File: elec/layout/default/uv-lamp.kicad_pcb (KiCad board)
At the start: 2 copper layers, 21 x 21 mm, 3 parts, among them U1 ?, U2 ?, U3 ?

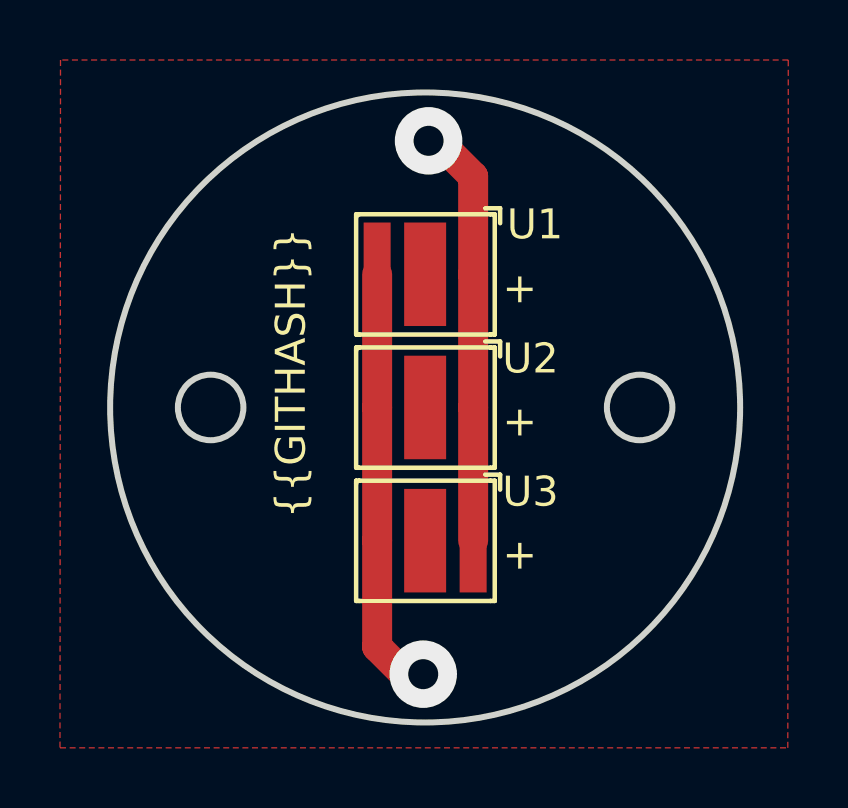
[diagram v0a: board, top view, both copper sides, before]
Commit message: readme
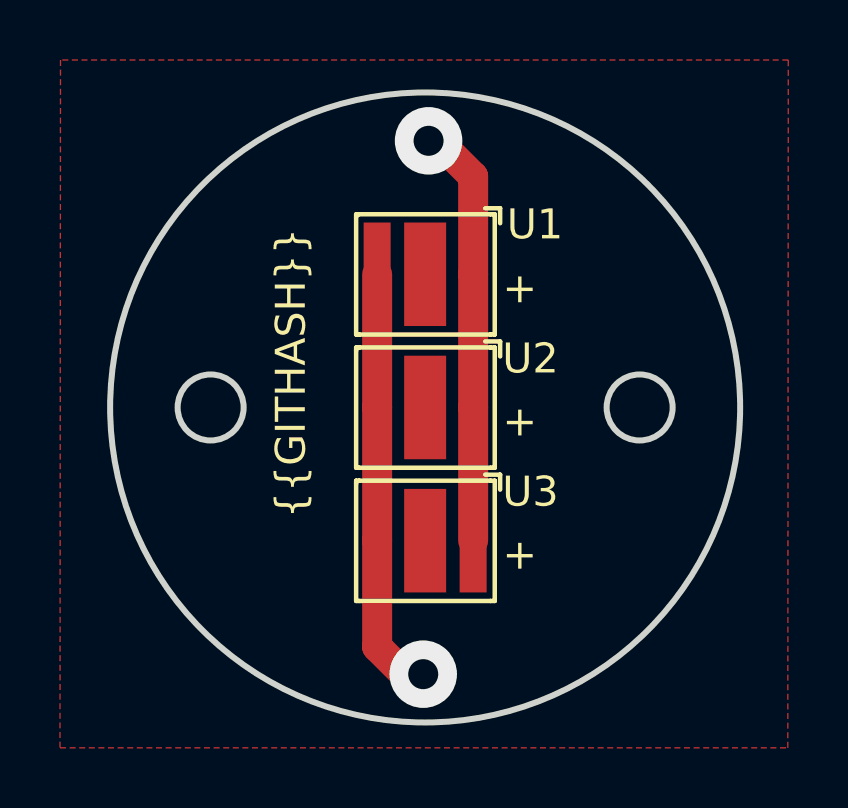
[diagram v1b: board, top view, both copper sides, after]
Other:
- outline, holes or cut-outs redrawn
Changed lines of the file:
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@@
 	(gr_circle
 		(center 155.04 86.31)
-		(end 156.132 86.31)
+		(end 156.14 86.31)
 		(stroke
 			(width 0.2)
@@
 	(gr_circle
 		(center 140.74 86.31)
-		(end 141.832 86.31)
+		(end 141.84 86.31)
 		(stroke
 			(width 0.2)
